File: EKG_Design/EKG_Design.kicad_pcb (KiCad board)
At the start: 2 copper layers, 41.4 x 22.6 mm, 55 parts, among them IC101 OPA2156IDGKR, IC102 OPA2156IDGKR, IC103 OPA2156IDGKR, IC104 INA826AIDR_/_SOIC8, J100 Conn_01x02_Pin, J101 Conn_01x02_Pin, J102 Conn_01x02_Pin, J103 Conn_01x02_Pin, J104 Conn_01x03_Pin, Q200 BC848C

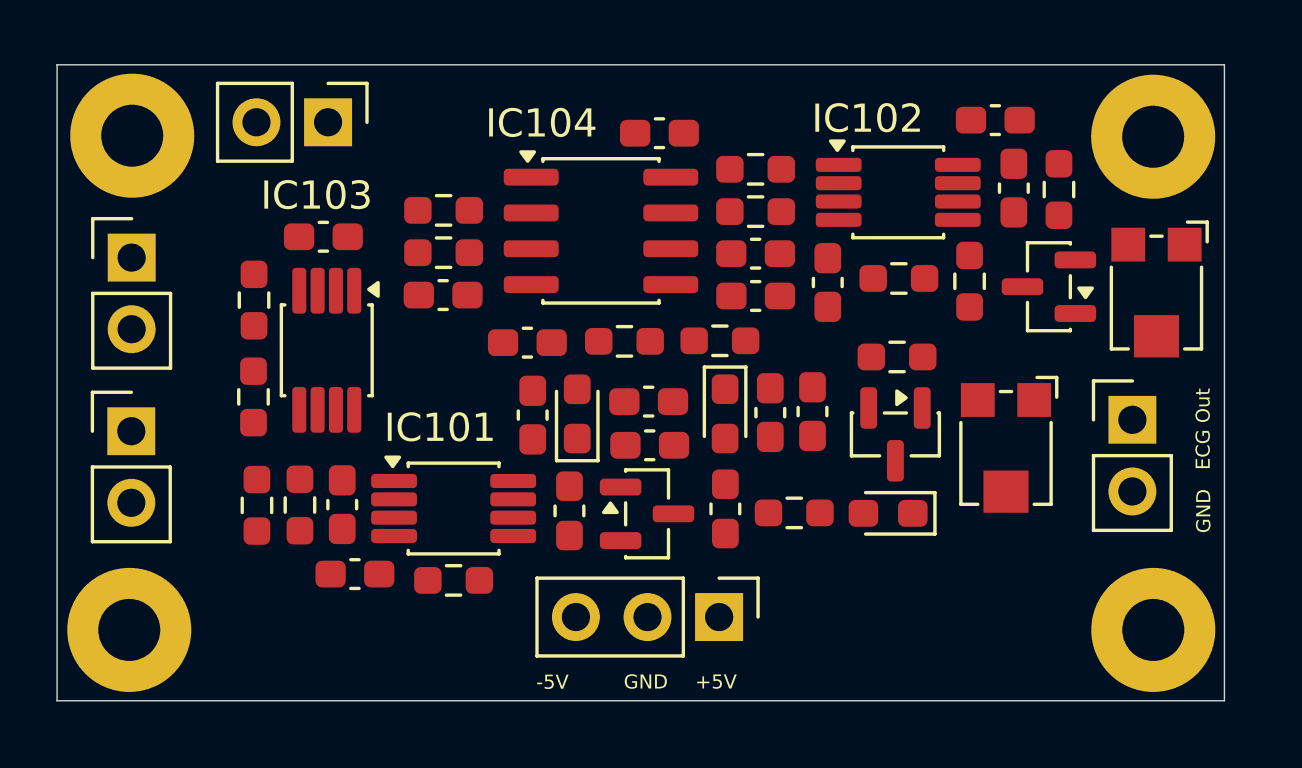
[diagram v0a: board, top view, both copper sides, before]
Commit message: Finished ECG Routing
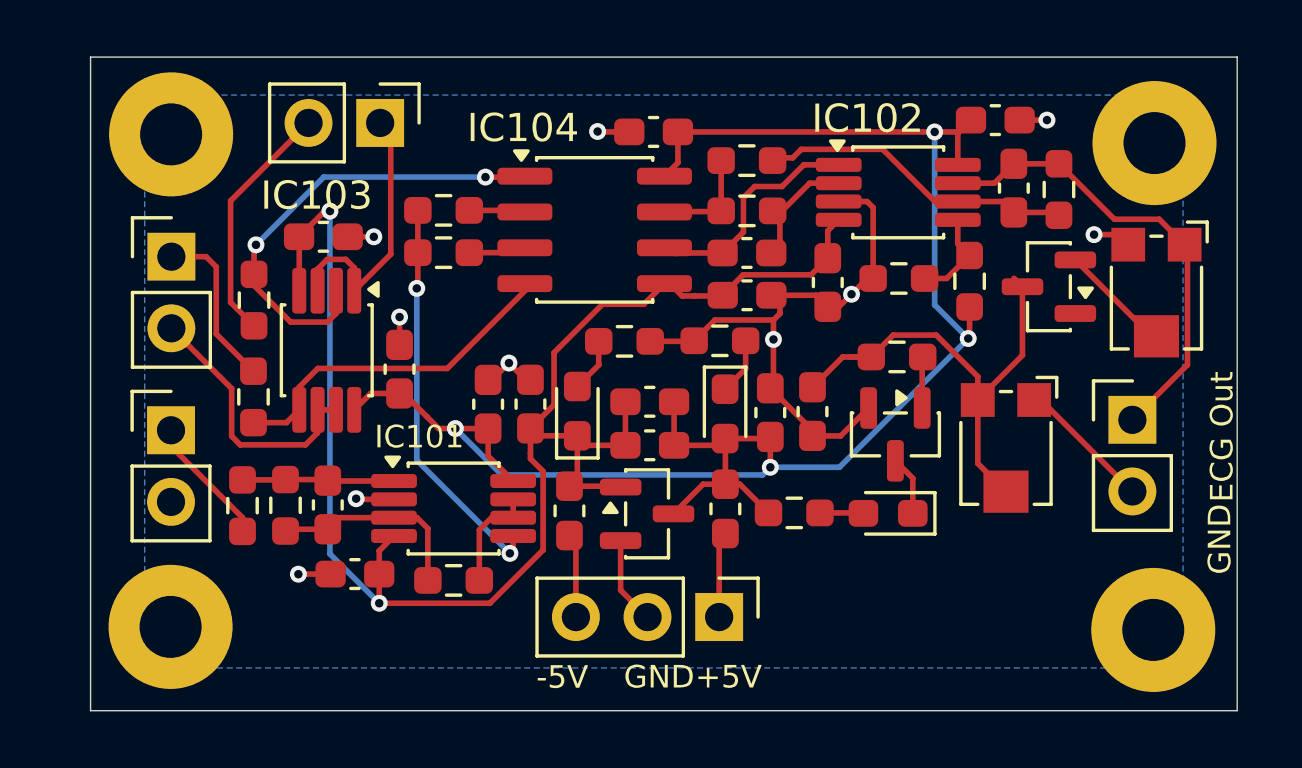
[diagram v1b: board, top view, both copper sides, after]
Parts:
- moved C104 4.63 mm to (103.0, 78.3), turned to 90 degrees
- moved C105 4.19 mm to (106.2, 79.5), turned to 90 degrees
- moved J100 1.85 mm to (102.3, 69.6)
- moved H102 1.47 mm to (94.9, 87.4)
- moved J101 1.41 mm to (94.9, 74.3)
- moved J102 1.41 mm to (94.9, 80.5)
- moved H103 1.38 mm to (94.9, 70.0)
- moved R108 0.51 mm to (99.0, 83.1)
- moved R109 0.51 mm to (97.4, 83.1)
- moved C102 0.51 mm to (100.5, 83.1)
- moved R102 0.44 mm to (115.3, 70.9)
- moved C106 0.40 mm to (107.7, 79.5)
- moved C100 0.31 mm to (115.3, 74.2)
- moved C107 0.31 mm to (115.3, 75.7)
- moved R103 0.31 mm to (115.3, 72.7)
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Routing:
- net 5V0_Analog: track 0.00 -> 63.1 mm, vias 0 -> 4
- net 5N0_Analog: track 0.00 -> 56.5 mm, vias 0 -> 2
- net GND: track 0.00 -> 38.8 mm, vias 0 -> 10
- net Net-(D200-C): track 0.00 -> 17.6 mm
- net /EKG-Details/EKG+: track 0.00 -> 16.6 mm, vias 0 -> 2
- net ECG_Out: track 0.00 -> 16.6 mm
- net /EKG-Details/VCM: track 0.00 -> 14.3 mm, vias 0 -> 2
- net /EKG-Details/EKG-: track 0.00 -> 12.4 mm
- net Net-(IC102B--): track 0.00 -> 11.2 mm
- net /EKG-Details/Shield+: track 0.00 -> 9.79 mm
- net /EKG-Details/Shield-: track 0.00 -> 9.53 mm
- net Net-(J100-Pin_2): track 0.00 -> 8.69 mm
- net Net-(IC104-Ref): track 0.00 -> 8.51 mm
- net Net-(IC101A-+): track 0.00 -> 7.24 mm
- net Net-(J101-Pin_1): track 0.00 -> 6.22 mm
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- added copper zone on B.Cu, net GND
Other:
- board size 41.4 x 22.6 mm -> 40.7 x 23.2 mm
